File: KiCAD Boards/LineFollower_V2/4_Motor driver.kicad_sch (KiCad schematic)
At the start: 2 parts, among them CN1 HC-2510-2A, CN2 HC-2510-2A

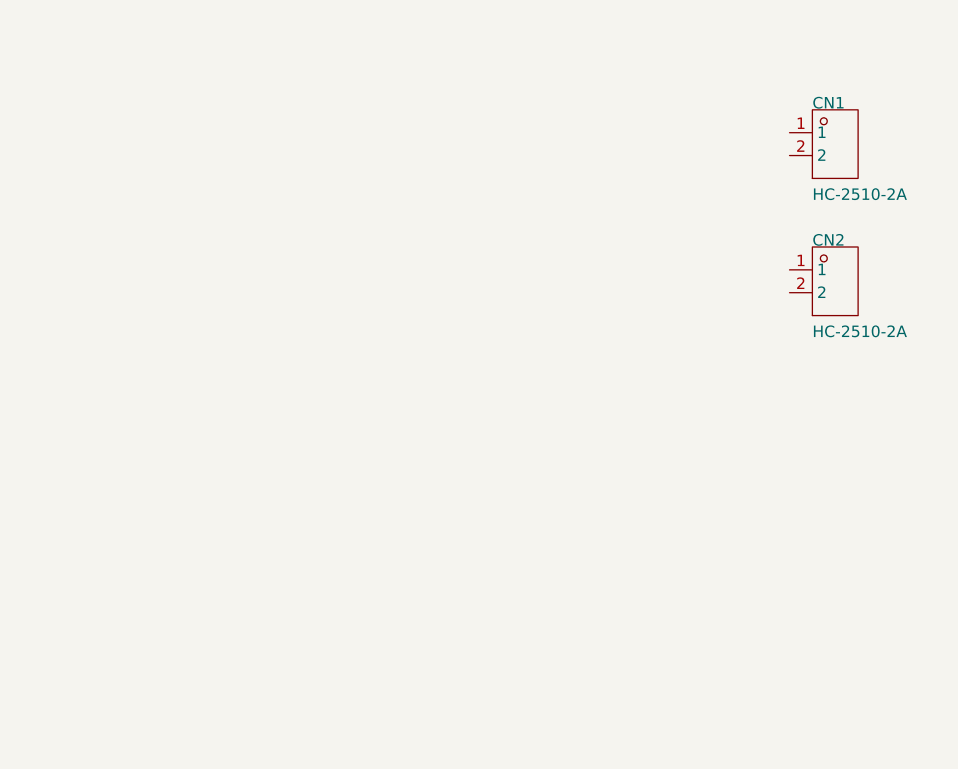
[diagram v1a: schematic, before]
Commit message: ZubyMakove
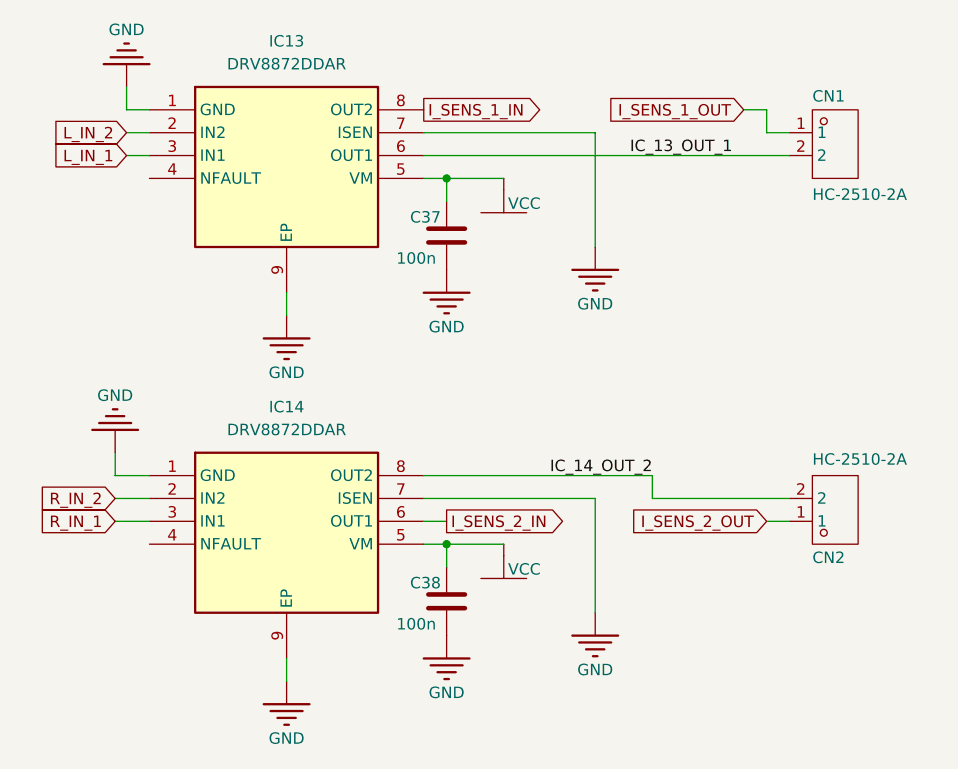
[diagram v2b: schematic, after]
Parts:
- added C37, C38: 100n, Capacitor_SMD:C_0603_1608Metric, symbol Device:C
- added IC13, IC14: DRV8872DDAR, SOIC127P600X170-9N, symbol M4JCI:DRV8872DDAR
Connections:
- net I_SENS_1_OUT: now reaches CN1.1
- net IC_13_OUT_1: now reaches CN1.2
- net IC_13_OUT_1: now also IC13.6 (OUT1)
- net I_SENS_2_OUT: now reaches CN2.1
- net IC_14_OUT_2: now reaches CN2.2
- net IC_14_OUT_2: now also IC14.8 (OUT2)
- new net GND: C37.1, C38.1, IC13.1 (GND), IC13.7 (ISEN), IC13.9 (EP), IC14.1 (GND), IC14.7 (ISEN), IC14.9 (EP)
- new net I_SENS_1_IN: IC13.8 (OUT2)
- new net I_SENS_2_IN: IC14.6 (OUT1)
- new net L_IN_1: IC13.3 (IN1)
- new net L_IN_2: IC13.2 (IN2)
- new net R_IN_1: IC14.3 (IN1)
- new net R_IN_2: IC14.2 (IN2)
- new net VCC: C37.2, C38.2, IC13.5 (VM), IC14.5 (VM)
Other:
- moved on the sheet: CN2
